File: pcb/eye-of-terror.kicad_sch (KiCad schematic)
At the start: 237 parts, among them J1 Conn_01x02_Socket, J2 G-Switch GT-USB-7055E, J3 Conn_01x04, J4 Conn_01x04, J5 Conn_01x03, J6 Conn_01x02_Socket, J7 Conn_01x02_Socket, J8 Conn_01x03, Q1 IPT020N10N3, Q10 ALS-PT19-315C/L177/TR8, Q11 ALS-PT19-315C/L177/TR8, Q12 ALS-PT19-315C/L177/TR8, Q13 ALS-PT19-315C/L177/TR8, Q14 ALS-PT19-315C/L177/TR8, Q15 ALS-PT19-315C/L177/TR8, Q16 ALS-PT19-315C/L177/TR8, Q17 NMOS, Q2 IPT020N10N3, Q3 IPT020N10N3, Q4 IPT020N10N3, Q5 IPT020N10N3, Q6 IPT020N10N3, Q7 ALS-PT19-315C/L177/TR8, Q8 ALS-PT19-315C/L177/TR8, Q9 ALS-PT19-315C/L177/TR8, SW1 SW_Push, SW2 SW_Push, U1 RP2350B, U2 TD1660, U3 AP63205WU-7, U4 LSM6DS3, U5 W25Q32JVSS, U7 DRV8353HRTAR, U8 ESD122DMXR, Y1 ABM8-272-T3

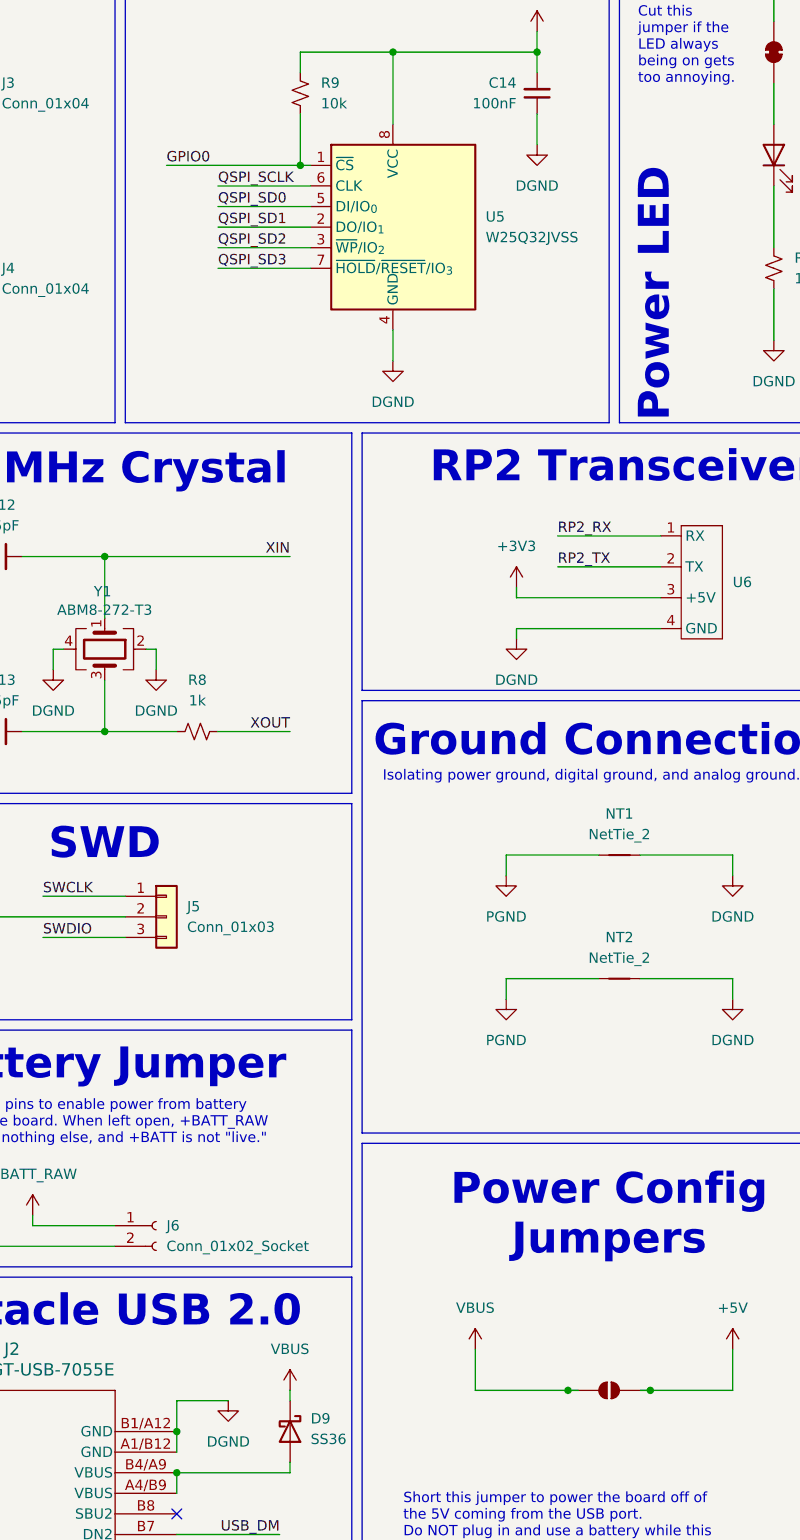
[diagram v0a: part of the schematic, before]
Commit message: WIP layout
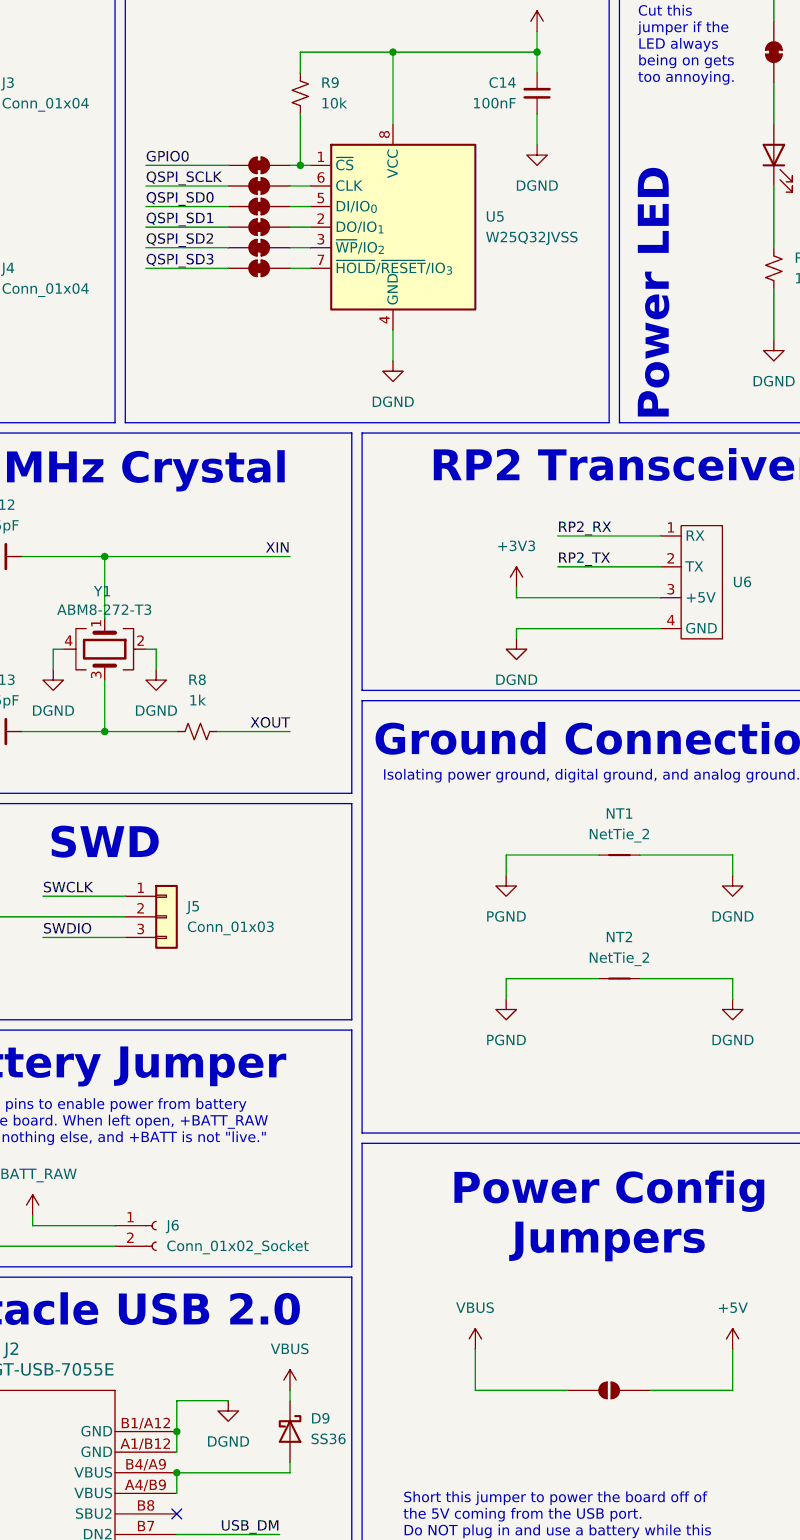
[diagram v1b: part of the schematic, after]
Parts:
- added JP19, JP20, JP21, JP22, JP23, JP24: SolderJumper_2_Bridged, Jumper:SolderJumper-2_P1.3mm_Bridged_RoundedPad1.0x1.5mm, symbol Jumper:SolderJumper_2_Bridged
- JP17: footprint Jumper:SolderJumper-2_P1.3mm_Bridged_RoundedPad1.0x1.5mm -> Jumper:SolderJumper-2_P1.3mm_Open_RoundedPad1.0x1.5mm
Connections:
- net GPIO0: now also JP19.1 (A); no longer R9.2, U5.1 (~{CS})
- net QSPI_SCLK: now also JP20.1 (A); no longer U5.6 (CLK)
- net QSPI_SD0: now also JP21.1 (A); no longer U5.5 (DI/IO_{0})
- net QSPI_SD1: now also JP22.1 (A); no longer U5.2 (DO/IO_{1})
- net QSPI_SD2: now also JP23.1 (A); no longer U5.3 (~{WP}/IO_{2})
- net QSPI_SD3: now also JP24.1 (A); no longer U5.7 (~{HOLD}/~{RESET}/IO_{3})
- new net: JP23.2 (B), U5.3 (~{WP}/IO_{2})
- new net: JP19.2 (B), R9.2, U5.1 (~{CS})
- new net: JP22.2 (B), U5.2 (DO/IO_{1})
- new net: JP20.2 (B), U5.6 (CLK)
- new net: JP21.2 (B), U5.5 (DI/IO_{0})
- new net: JP24.2 (B), U5.7 (~{HOLD}/~{RESET}/IO_{3})

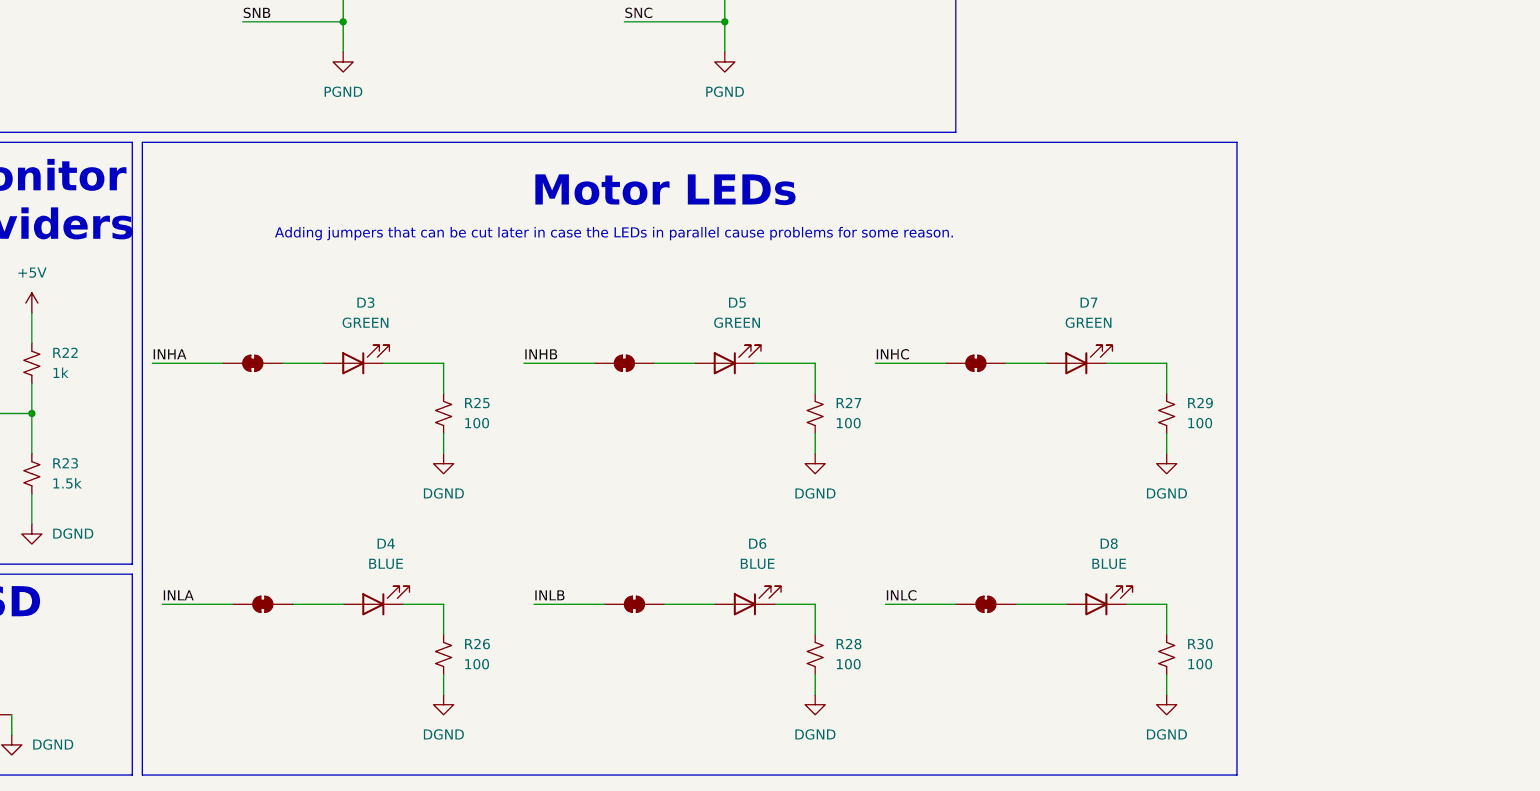
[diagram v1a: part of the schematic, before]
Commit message: WIP layout almost done
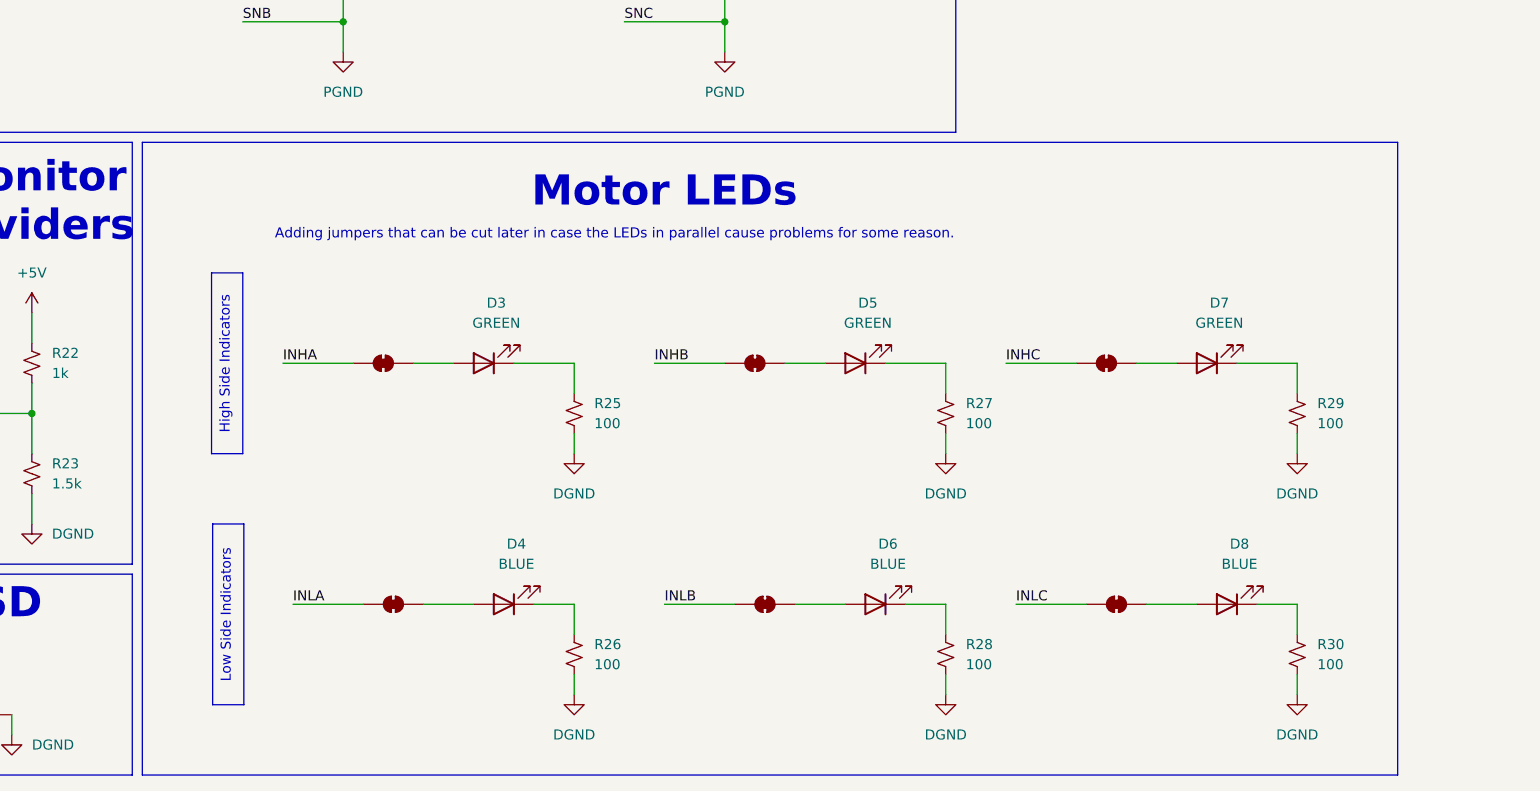
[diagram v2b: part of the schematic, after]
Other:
- moved on the sheet: D3, D4, D5, D6, D7, D8, R25, R26, R27, R28, R29, R30
